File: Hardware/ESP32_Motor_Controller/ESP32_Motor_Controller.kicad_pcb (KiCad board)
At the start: 4 copper layers, 65 x 56.4 mm, 154 parts, among them IC501 MT6701CT-AKD, J101 XT30PW-M, J102 XT30PW-M, J501 Hall Encoder, J502 CAN1, J503 CAN2, Q1 XRS80P06F, Q401 FH4008GS, Q402 FH4008GS, Q403 FH4008GS, Q404 FH4008GS, Q405 FH4008GS, Q406 FH4008GS, SW1 TS-1088-AR02016, SW2 TS-1088-AR02016, U2 TLV75733PDBV, U301 DRV8302DCAR, U501 BMI270, U502 MCP2551-I_SN

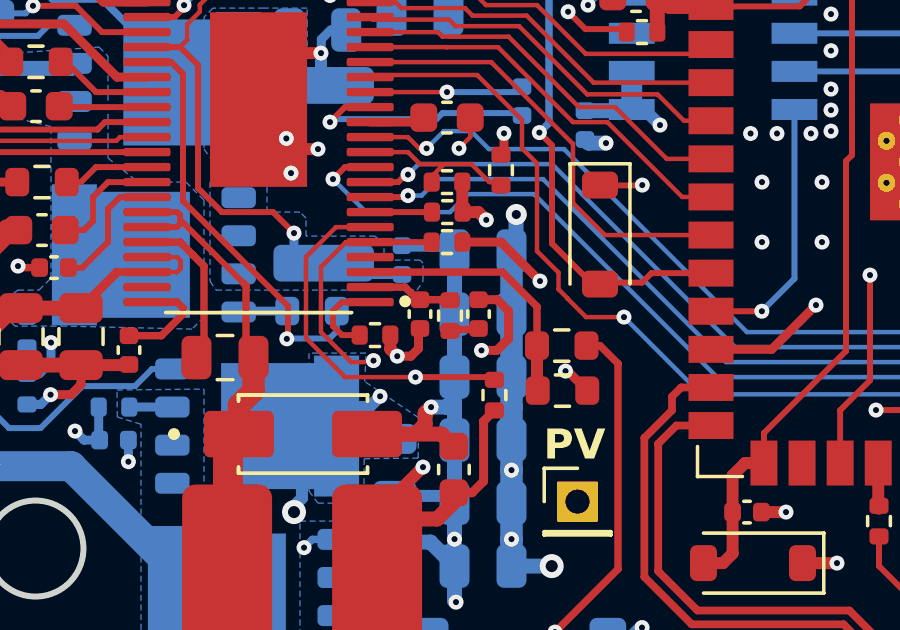
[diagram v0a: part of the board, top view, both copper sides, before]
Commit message: Buck Components Update
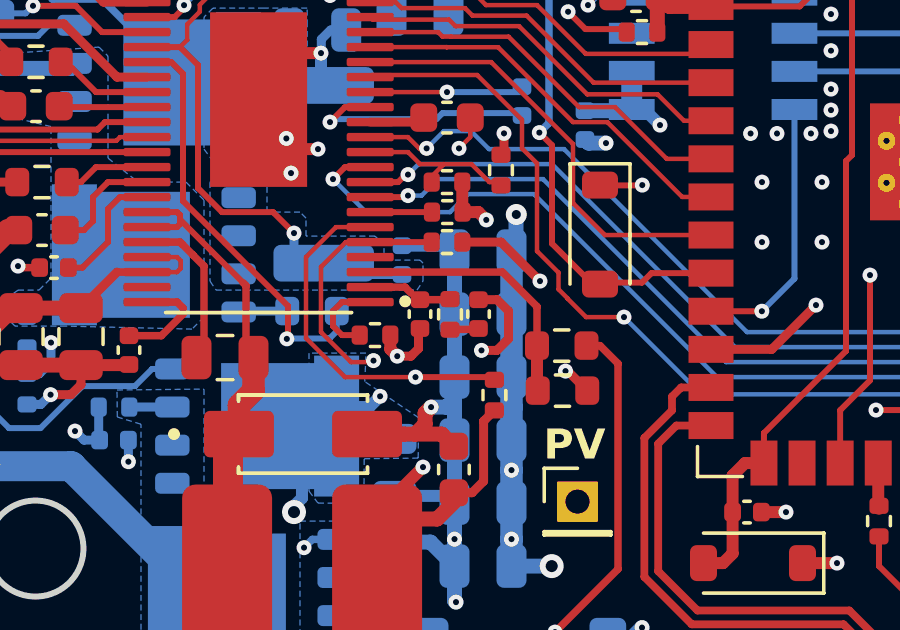
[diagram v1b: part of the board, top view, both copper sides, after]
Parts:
- C317: value 1.5nF -> 15pF
- C318: value 36pF -> 1nF
- C319: value 47uF -> 22uF
- C506: value 0.1uF -> 1uF
- R306: value 15k -> 86.6k
- R308: value 3.3k -> 10k
- R309: value 10k -> 52.3k
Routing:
- net AGND: vias 164 -> 165
- net 5V: vias 12 -> 11
